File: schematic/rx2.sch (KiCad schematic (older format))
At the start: 61 parts, among them J4 AudioJack3, Q11 2N3904, Q12 2N3904, Q13 2N7000, T2 FT37-43, U6 ADE-1, U7 L7809, U8 LM386, Y2 9 MHz, Y3 9 MHz, Y4 9 MHz, Y5 9 MHz, Y6 9 MHz

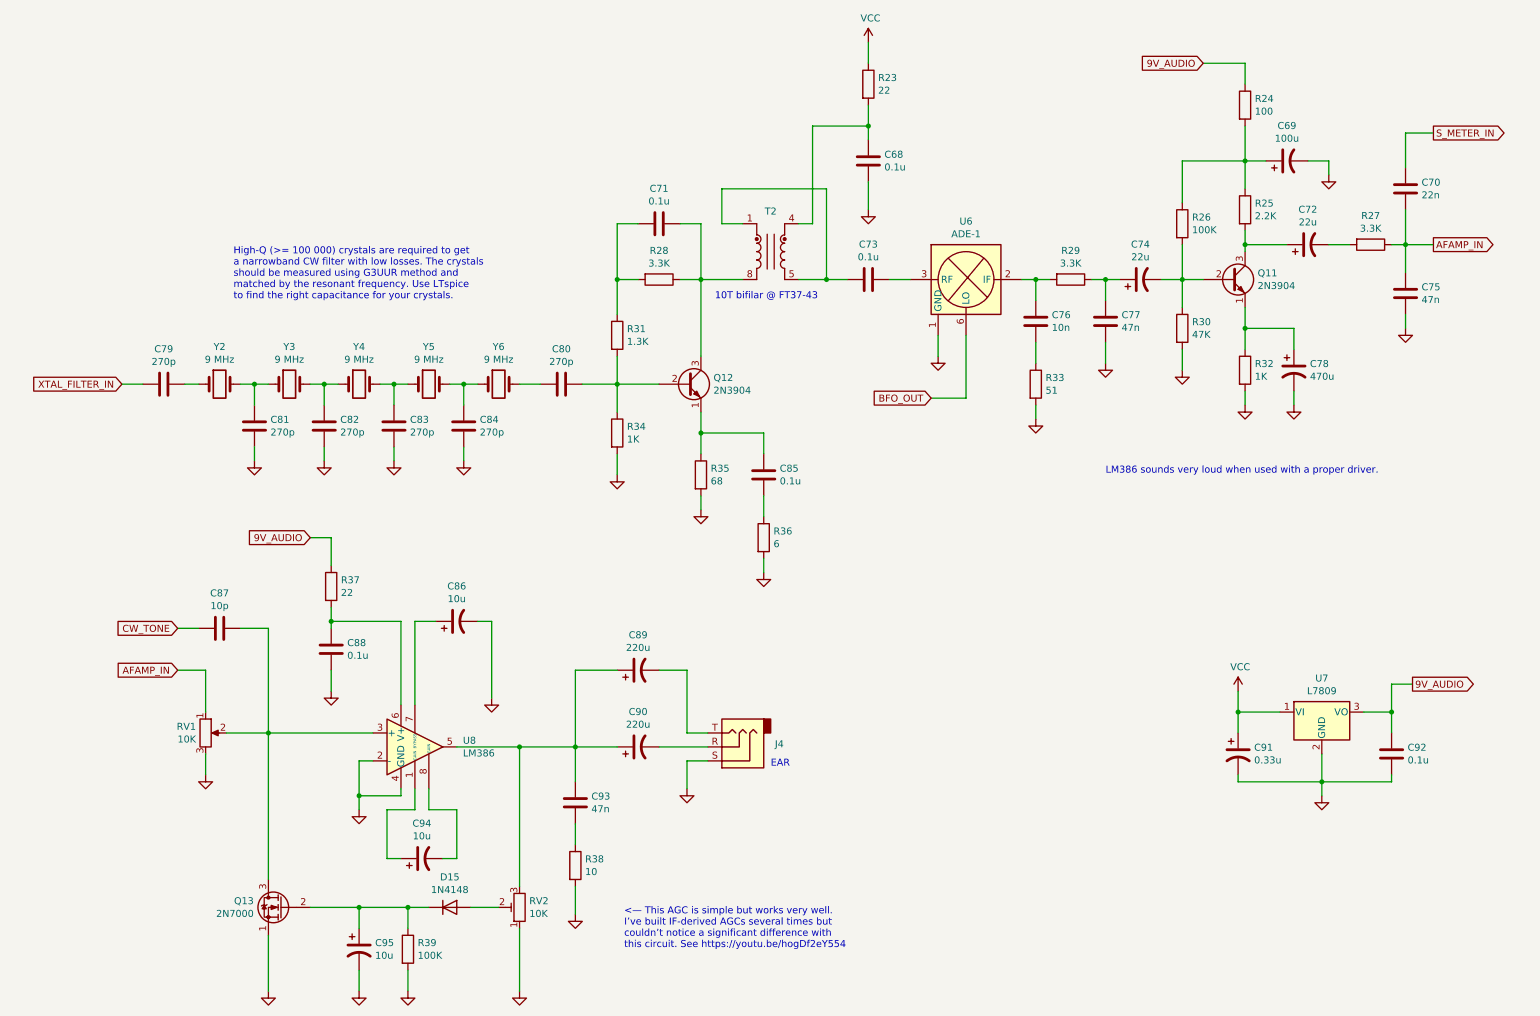
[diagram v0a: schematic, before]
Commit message: Some minor tweaks
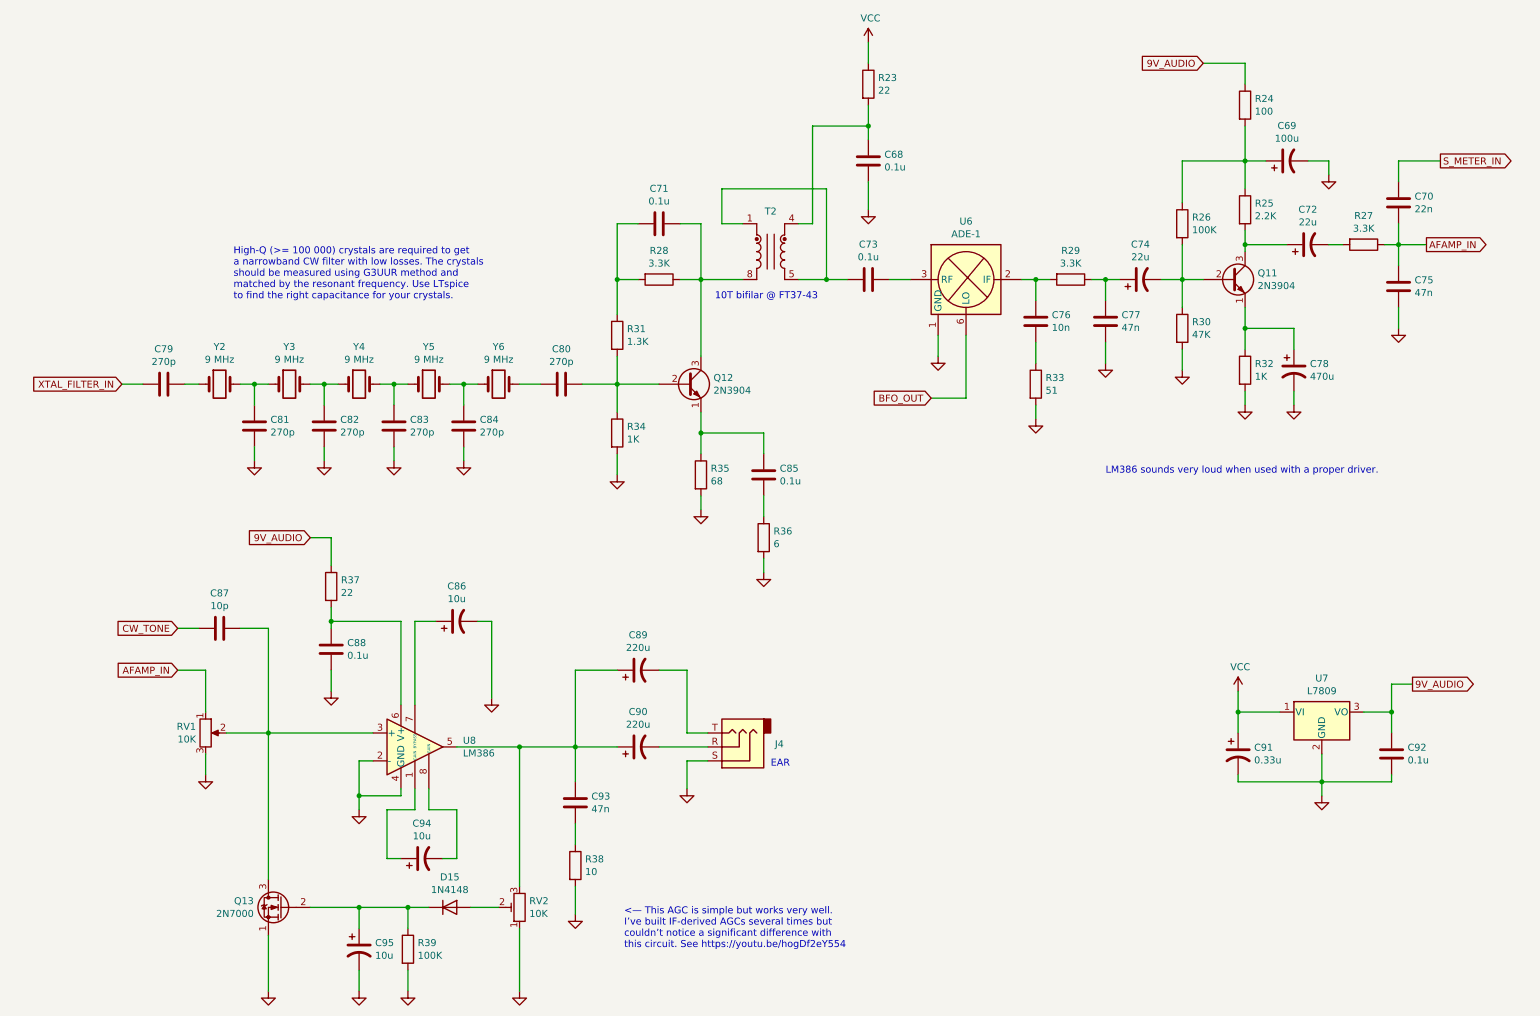
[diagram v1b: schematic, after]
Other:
- moved on the sheet: C70
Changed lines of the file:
@@
 	0    -1   -1   0
 $EndComp
-$Comp
-L Device:R R?
-U 1 1 62D7544D
-P 10150 2200
-AR Path="/62C0C022/62D7544D" Ref="R?"  Part="1"
-AR Path="/62CCEF11/62D7544D" Ref="R27"  Part="1"
-F 0 "R27" V 9943 2200 50  0000 C CNN
-F 1 "3.3K" V 10034 2200 50  0000 C CNN
-F 2 "" V 10080 2200 50  0001 C CNN
-F 3 "~" H 10150 2200 50  0001 C CNN
-	1    10150 2200
-	0    1    1    0
-$EndComp
-$Comp
-L Device:C C75
-U 1 1 62D7598D
-P 10400 2550
-F 0 "C75" H 10515 2596 50  0000 L CNN
-F 1 "47n" H 10515 2505 50  0000 L CNN
-F 2 "" H 10438 2400 50  0001 C CNN
-F 3 "~" H 10400 2550 50  0001 C CNN
-	1    10400 2550
-	1    0    0    -1
-$EndComp
-Text GLabel 10600 2200 2    50   Output ~ 0
+Text GLabel 10550 2200 2    50   Output ~ 0
 AFAMP_IN
-$Comp
-L power:GND #PWR?
-U 1 1 62D76BC9
-P 10400 2800
-AR Path="/62C0C022/62D76BC9" Ref="#PWR?"  Part="1"
-AR Path="/62CCEF11/62D76BC9" Ref="#PWR0104"  Part="1"
-F 0 "#PWR0104" H 10400 2550 50  0001 C CNN
-F 1 "GND" H 10405 2627 50  0001 C CNN
-F 2 "" H 10400 2800 50  0001 C CNN
-F 3 "" H 10400 2800 50  0001 C CNN
-	1    10400 2800
-	1    0    0    -1
-$EndComp
 Wire Wire Line
 	7650 2450 7750 2450
@@
 Wire Wire Line
 	9250 2200 9250 2100
-Wire Wire Line
-	9850 2200 10000 2200
-Wire Wire Line
-	10300 2200 10400 2200
-Wire Wire Line
-	10400 2200 10400 2400
-Connection ~ 10400 2200
-Wire Wire Line
-	10400 2200 10600 2200
-Wire Wire Line
-	10400 2700 10400 2800
 Wire Wire Line
 	9250 2950 9250 2800
@@
 Wire Wire Line
 	1800 5550 1800 5250
-Wire Wire Line
-	1800 5250 1600 5250
 $Comp
 L Amplifier_Audio:LM386 U8
@@
 Text Notes 2000 2600 0    50   ~ 0
 High-Q (>= 100 000) crystals are required to get\na narrowband CW filter with low losses. The crystals\nshould be measured using G3UUR method and\nmatched by the resonant frequency. Use LTspice\nto find the right capacitance for your crystals.
-Text GLabel 10600 1400 2    50   Output ~ 0
+Text GLabel 10650 1600 2    50   Output ~ 0
 S_METER_IN
 $Comp
 L Device:C C70
 U 1 1 6310FC29
-P 10400 1800
-F 0 "C70" H 10515 1846 50  0000 L CNN
-F 1 "22n" H 10515 1755 50  0000 L CNN
-F 2 "" H 10438 1650 50  0001 C CNN
-F 3 "~" H 10400 1800 50  0001 C CNN
-	1    10400 1800
-	1    0    0    -1
-$EndComp
-Wire Wire Line
-	10400 2200 10400 1950
-Wire Wire Line
-	10400 1650 10400 1400
-Wire Wire Line
-	10400 1400 10600 1400
+P 10350 1900
+F 0 "C70" H 10465 1946 50  0000 L CNN
+F 1 "22n" H 10465 1855 50  0000 L CNN
+F 2 "" H 10388 1750 50  0001 C CNN
+F 3 "~" H 10350 1900 50  0001 C CNN
+	1    10350 1900
+	1    0    0    -1
+$EndComp
+Wire Wire Line
+	10350 2200 10350 2050
+Wire Wire Line
+	10350 1750 10350 1600
+Wire Wire Line
+	10350 1600 10650 1600
+Wire Wire Line
+	1600 5250 1800 5250
+$Comp
+L Device:R R?
+U 1 1 62FE865F
+P 10100 2200
+AR Path="/62C0C022/62FE865F" Ref="R?"  Part="1"
+AR Path="/62CCEF11/62FE865F" Ref="R27"  Part="1"
+F 0 "R27" V 9893 2200 50  0000 C CNN
+F 1 "3.3K" V 9984 2200 50  0000 C CNN
+F 2 "" V 10030 2200 50  0001 C CNN
+F 3 "~" H 10100 2200 50  0001 C CNN
+	1    10100 2200
+	0    1    1    0
+$EndComp
+$Comp
+L Device:C C75
+U 1 1 62FE8669
+P 10350 2500
+F 0 "C75" H 10465 2546 50  0000 L CNN
+F 1 "47n" H 10465 2455 50  0000 L CNN
+F 2 "" H 10388 2350 50  0001 C CNN
+F 3 "~" H 10350 2500 50  0001 C CNN
+	1    10350 2500
+	1    0    0    -1
+$EndComp
+$Comp
+L power:GND #PWR?
+U 1 1 62FE8673
+P 10350 2800
+AR Path="/62C0C022/62FE8673" Ref="#PWR?"  Part="1"
+AR Path="/62CCEF11/62FE8673" Ref="#PWR0104"  Part="1"
+F 0 "#PWR0104" H 10350 2550 50  0001 C CNN
+F 1 "GND" H 10355 2627 50  0001 C CNN
+F 2 "" H 10350 2800 50  0001 C CNN
+F 3 "" H 10350 2800 50  0001 C CNN
+	1    10350 2800
+	1    0    0    -1
+$EndComp
+Wire Wire Line
+	10250 2200 10350 2200
+Wire Wire Line
+	10350 2200 10350 2350
+Connection ~ 10350 2200
+Wire Wire Line
+	10350 2650 10350 2800
+Wire Wire Line
+	9950 2200 9850 2200
+Wire Wire Line
+	10350 2200 10550 2200
 $EndSCHEMATC
